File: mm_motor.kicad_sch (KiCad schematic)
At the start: 1 part, among them M1 N20_encoder

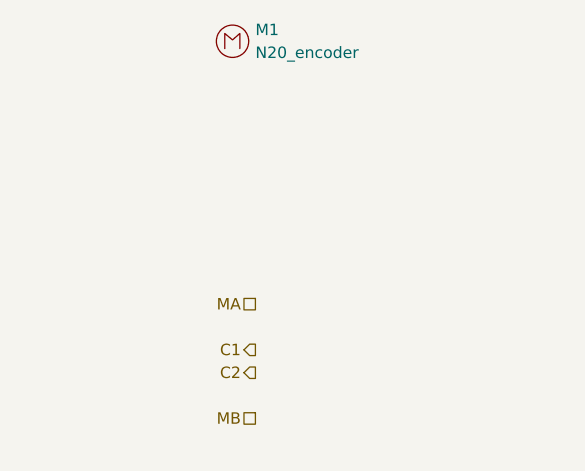
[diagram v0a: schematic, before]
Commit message: tp2
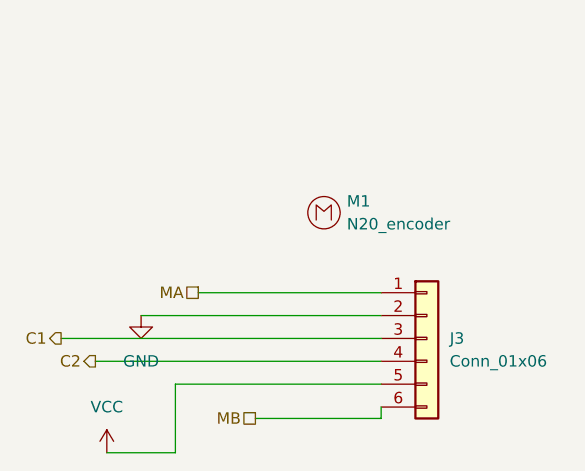
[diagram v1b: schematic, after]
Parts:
- added J3: Conn_01x06, symbol Connector_Generic:Conn_01x06
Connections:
- net C1: now also J3.3 (Pin_3)
- net C2: now also J3.4 (Pin_4)
- net MA: now also J3.1 (Pin_1)
- net MB: now also J3.6 (Pin_6)
- new net GND: J3.2 (Pin_2)
- new net VCC: J3.5 (Pin_5)
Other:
- moved on the sheet: M1
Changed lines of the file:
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@@
 (kicad_sch (version 20230121) (generator eeschema)
   (paper "A4")
-  (hierarchical_label "C1" (shape output) (at 118.11 91.44 180) (fields_autoplaced)
+  (wire (pts (xy 100.33 92.71) (xy 132.08 92.71))
+    (stroke (width 0) (type default))
+  )
+  (wire (pts (xy 101.6 102.87) (xy 109.22 102.87))
+    (stroke (width 0) (type default))
+  )
+  (wire (pts (xy 109.22 95.25) (xy 132.08 95.25))
+    (stroke (width 0) (type default))
+  )
+  (wire (pts (xy 132.08 99.06) (xy 132.08 97.79))
+    (stroke (width 0) (type default))
+  )
+  (wire (pts (xy 111.76 85.09) (xy 132.08 85.09))
+    (stroke (width 0) (type default))
+  )
+  (wire (pts (xy 118.11 99.06) (xy 132.08 99.06))
+    (stroke (width 0) (type default))
+  )
+  (wire (pts (xy 105.41 87.63) (xy 132.08 87.63))
+    (stroke (width 0) (type default))
+  )
+  (wire (pts (xy 96.52 90.17) (xy 132.08 90.17))
+    (stroke (width 0) (type default))
+  )
+  (wire (pts (xy 109.22 102.87) (xy 109.22 95.25))
+    (stroke (width 0) (type default))
+  )
+  (hierarchical_label "C1" (shape output) (at 96.52 90.17 180) (fields_autoplaced)
     (effects (font (size 1.27 1.27)) (justify right))
   )
-  (hierarchical_label "C2" (shape output) (at 118.11 93.98 180) (fields_autoplaced)
+  (hierarchical_label "C2" (shape output) (at 100.33 92.71 180) (fields_autoplaced)
     (effects (font (size 1.27 1.27)) (justify right))
   )
@@
     (effects (font (size 1.27 1.27)) (justify right))
   )
-  (hierarchical_label "MA" (shape passive) (at 118.11 86.36 180) (fields_autoplaced)
+  (hierarchical_label "MA" (shape passive) (at 111.76 85.09 180) (fields_autoplaced)
     (effects (font (size 1.27 1.27)) (justify right))
   )
-  (symbol (lib_id "minimouse:N20_w_encoder") (at 115.57 57.15 0) (unit 1)
+  (symbol (lib_id "Connector_Generic:Conn_01x06") (at 137.16 90.17 0) (unit 1)
     (in_bom yes) (on_board yes) (dnp no) (fields_autoplaced)
-    (property "Reference" "M1" (at 118.11 55.88 0)
+    (property "Reference" "J3" (at 139.7 90.17 0)
       (effects (font (size 1.27 1.27)) (justify left))
     )
-    (property "Value" "N20_encoder" (at 118.11 58.42 0)
+    (property "Value" "Conn_01x06" (at 139.7 92.71 0)
       (effects (font (size 1.27 1.27)) (justify left))
     )
-    (property "Footprint" "minimouse:N20_with_encoder" (at 118.11 53.34 0)
+    (property "Footprint" "" (at 137.16 90.17 0)
       (effects (font (size 1.27 1.27)) hide)
     )
-    (property "Datasheet" "" (at 115.57 57.15 0)
+    (property "Datasheet" "~" (at 137.16 90.17 0)
+      (effects (font (size 1.27 1.27)) hide)
+    )
+    (pin "3")
+    (pin "4")
+    (pin "5")
+    (pin "6")
+    (pin "2")
+    (pin "1")
+    (instances
+      (project "minimouse"
+        (path "/d8fa4cba-2469-4231-847f-065b6b829f44/7f113667-692a-4f4d-b16f-621d32f3f136"
+          (reference "J3") (unit 1)
+        )
+        (path "/d8fa4cba-2469-4231-847f-065b6b829f44/3975acd0-18ad-47bc-9ce1-d8c4d864aafe"
+          (reference "J4") (unit 1)
+        )
+      )
+    )
+  )
+  (symbol (lib_id "power:VCC") (at 101.6 102.87 0) (unit 1)
+    (in_bom yes) (on_board yes) (dnp no) (fields_autoplaced)
+    (property "Reference" "#PWR022" (at 101.6 106.68 0)
+      (effects (font (size 1.27 1.27)) hide)
+    )
+    (property "Value" "VCC" (at 101.6 97.79 0)
+      (effects (font (size 1.27 1.27)))
+    )
+    (property "Footprint" "" (at 101.6 102.87 0)
+      (effects (font (size 1.27 1.27)) hide)
+    )
+    (property "Datasheet" "" (at 101.6 102.87 0)
+      (effects (font (size 1.27 1.27)) hide)
+    )
+    (pin "1")
+    (instances
+      (project "minimouse"
+        (path "/d8fa4cba-2469-4231-847f-065b6b829f44/3975acd0-18ad-47bc-9ce1-d8c4d864aafe"
+          (reference "#PWR022") (unit 1)
+        )
+        (path "/d8fa4cba-2469-4231-847f-065b6b829f44/7f113667-692a-4f4d-b16f-621d32f3f136"
+          (reference "#PWR021") (unit 1)
+        )
+      )
+    )
+  )
+  (symbol (lib_id "minimouse:N20_w_encoder") (at 125.73 76.2 0) (unit 1)
+    (in_bom yes) (on_board yes) (dnp no) (fields_autoplaced)
+    (property "Reference" "M1" (at 128.27 74.93 0)
+      (effects (font (size 1.27 1.27)) (justify left))
+    )
+    (property "Value" "N20_encoder" (at 128.27 77.47 0)
+      (effects (font (size 1.27 1.27)) (justify left))
+    )
+    (property "Footprint" "minimouse:N20_with_encoder" (at 128.27 72.39 0)
+      (effects (font (size 1.27 1.27)) hide)
+    )
+    (property "Datasheet" "" (at 125.73 76.2 0)
       (effects (font (size 1.27 1.27)) hide)
     )
@@
         )
       )
+    )
+  )
+  (symbol (lib_id "power:GND") (at 105.41 87.63 0) (unit 1)
+    (in_bom yes) (on_board yes) (dnp no) (fields_autoplaced)
+    (property "Reference" "#PWR020" (at 105.41 93.98 0)
+      (effects (font (size 1.27 1.27)) hide)
+    )
+    (property "Value" "GND" (at 105.41 92.71 0)
+      (effects (font (size 1.27 1.27)))
+    )
+    (property "Footprint" "" (at 105.41 87.63 0)
+      (effects (font (size 1.27 1.27)) hide)
+    )
+    (property "Datasheet" "" (at 105.41 87.63 0)
+      (effects (font (size 1.27 1.27)) hide)
+    )
+    (pin "1")
+    (instances
+      (project "minimouse"
+        (path "/d8fa4cba-2469-4231-847f-065b6b829f44/3975acd0-18ad-47bc-9ce1-d8c4d864aafe"
+          (reference "#PWR020") (unit 1)
+        )
+        (path "/d8fa4cba-2469-4231-847f-065b6b829f44/7f113667-692a-4f4d-b16f-621d32f3f136"
+          (reference "#PWR019") (unit 1)
+        )
+      )
